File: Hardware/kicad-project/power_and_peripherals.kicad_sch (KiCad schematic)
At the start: 42 parts, among them CN1 Conn_02x08_Odd_Even, CN2 Conn_02x15_Odd_Even, CN3 Conn_02x17_Odd_Even, CN4 Conn_02x10_Odd_Even, J1 Conn_01x02, J2 UART, J3 Torque, J4 Stepper supply, J5 Brake, Q1 Q_NMOS_DGS, Q2 Q_NMOS_DGS, U1 LM7812_TO220, U2 L7805

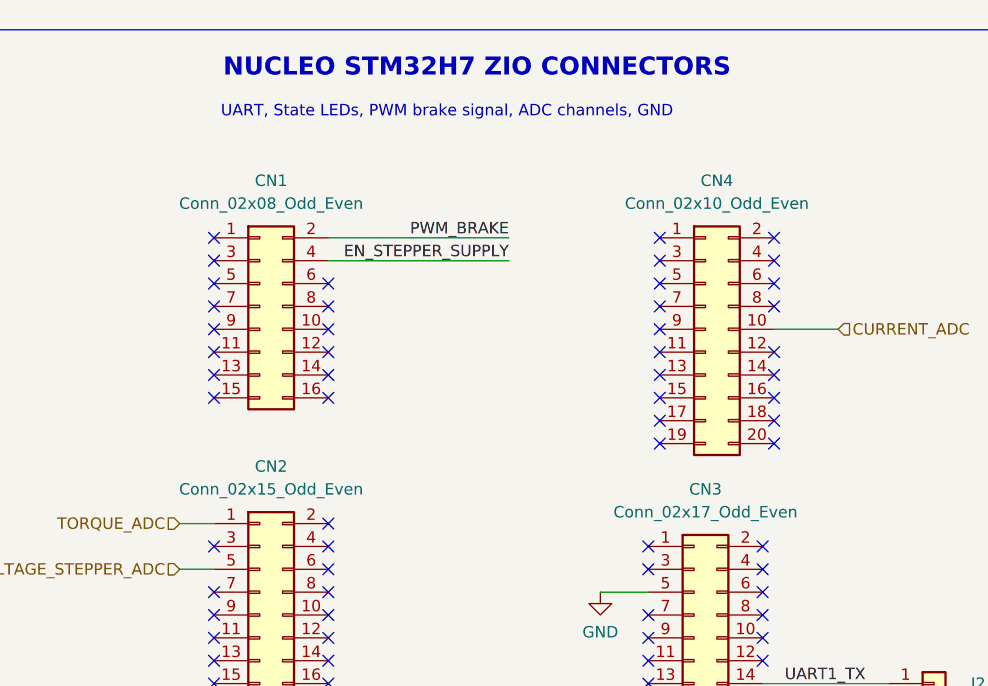
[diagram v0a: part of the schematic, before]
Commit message: hw: add note to layout and add pdf
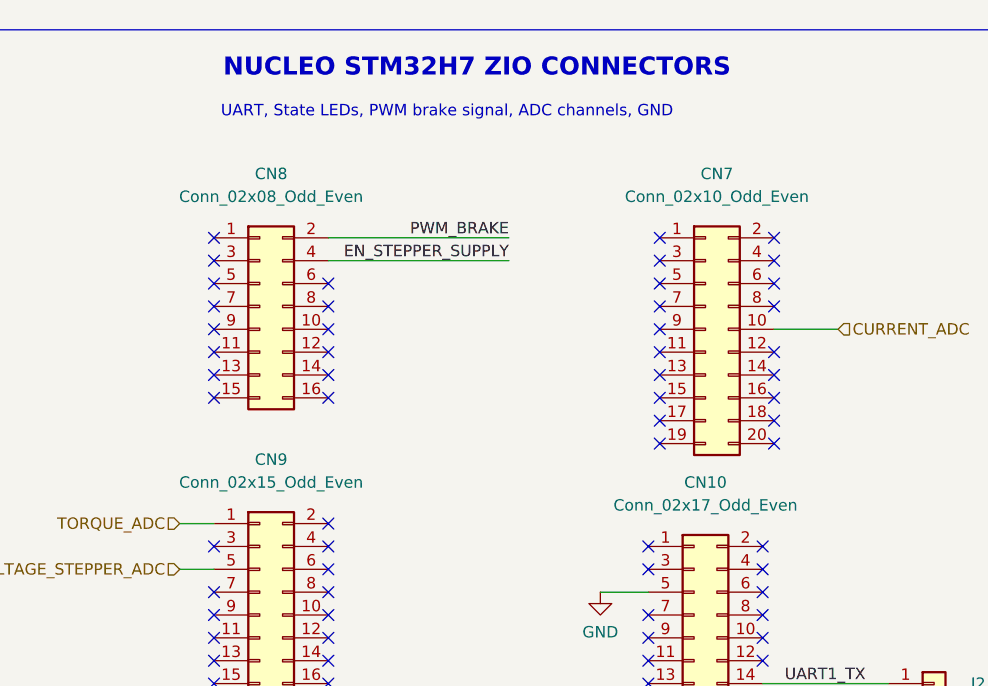
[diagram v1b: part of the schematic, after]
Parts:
- renumbered CN3 to CN10, CN4 to CN7, CN1 to CN8, CN2 to CN9
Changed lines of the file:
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@@
   (symbol (lib_id "Connector_Generic:Conn_02x08_Odd_Even") (at 51.308 104.902 0) (unit 1)
     (in_bom yes) (on_board yes) (fields_autoplaced)
-    (property "Reference" "CN1" (id 0) (at 52.578 90.932 0))
-    (property "Value" "Conn_02x08_Odd_Even" (id 1) (at 52.578 93.472 0))
+    (property "Reference" "CN8" (id 0) (at 52.578 90.17 0))
+    (property "Value" "Conn_02x08_Odd_Even" (id 1) (at 52.578 92.71 0))
     (property "Footprint" "Connector_PinHeader_2.54mm:PinHeader_2x08_P2.54mm_Vertical" (id 2) (at 51.308 104.902 0)
       (effects (font (size 1.27 1.27)) hide)
@@
   (symbol (lib_id "Connector_Generic:Conn_02x15_Odd_Even") (at 51.308 146.812 0) (unit 1)
     (in_bom yes) (on_board yes) (fields_autoplaced)
-    (property "Reference" "CN2" (id 0) (at 52.578 122.682 0))
-    (property "Value" "Conn_02x15_Odd_Even" (id 1) (at 52.578 125.222 0))
+    (property "Reference" "CN9" (id 0) (at 52.578 121.92 0))
+    (property "Value" "Conn_02x15_Odd_Even" (id 1) (at 52.578 124.46 0))
     (property "Footprint" "Connector_PinHeader_2.54mm:PinHeader_2x15_P2.54mm_Vertical" (id 2) (at 51.308 146.812 0)
       (effects (font (size 1.27 1.27)) hide)
@@
   (symbol (lib_id "Connector_Generic:Conn_02x17_Odd_Even") (at 99.568 151.892 0) (unit 1)
     (in_bom yes) (on_board yes) (fields_autoplaced)
-    (property "Reference" "CN3" (id 0) (at 100.838 125.222 0))
-    (property "Value" "Conn_02x17_Odd_Even" (id 1) (at 100.838 127.762 0))
+    (property "Reference" "CN10" (id 0) (at 100.838 124.46 0))
+    (property "Value" "Conn_02x17_Odd_Even" (id 1) (at 100.838 127 0))
     (property "Footprint" "Connector_PinHeader_2.54mm:PinHeader_2x17_P2.54mm_Vertical" (id 2) (at 99.568 151.892 0)
       (effects (font (size 1.27 1.27)) hide)
@@
   (symbol (lib_id "Connector_Generic:Conn_02x10_Odd_Even") (at 100.838 107.442 0) (unit 1)
     (in_bom yes) (on_board yes) (fields_autoplaced)
-    (property "Reference" "CN4" (id 0) (at 102.108 90.932 0))
-    (property "Value" "Conn_02x10_Odd_Even" (id 1) (at 102.108 93.472 0))
+    (property "Reference" "CN7" (id 0) (at 102.108 90.17 0))
+    (property "Value" "Conn_02x10_Odd_Even" (id 1) (at 102.108 92.71 0))
     (property "Footprint" "Connector_PinHeader_2.54mm:PinHeader_2x10_P2.54mm_Vertical" (id 2) (at 100.838 107.442 0)
       (effects (font (size 1.27 1.27)) hide)
